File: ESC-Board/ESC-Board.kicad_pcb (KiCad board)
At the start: 2 copper layers, 17.1 x 32 mm, 26 parts, among them J1 Molex, J2 Molex, J3 XT_60, U1 ESC:Blue_ESC, U2 ESC:Blue_ESC, U3 ESC:Blue_ESC, U4 ESC:Blue_ESC

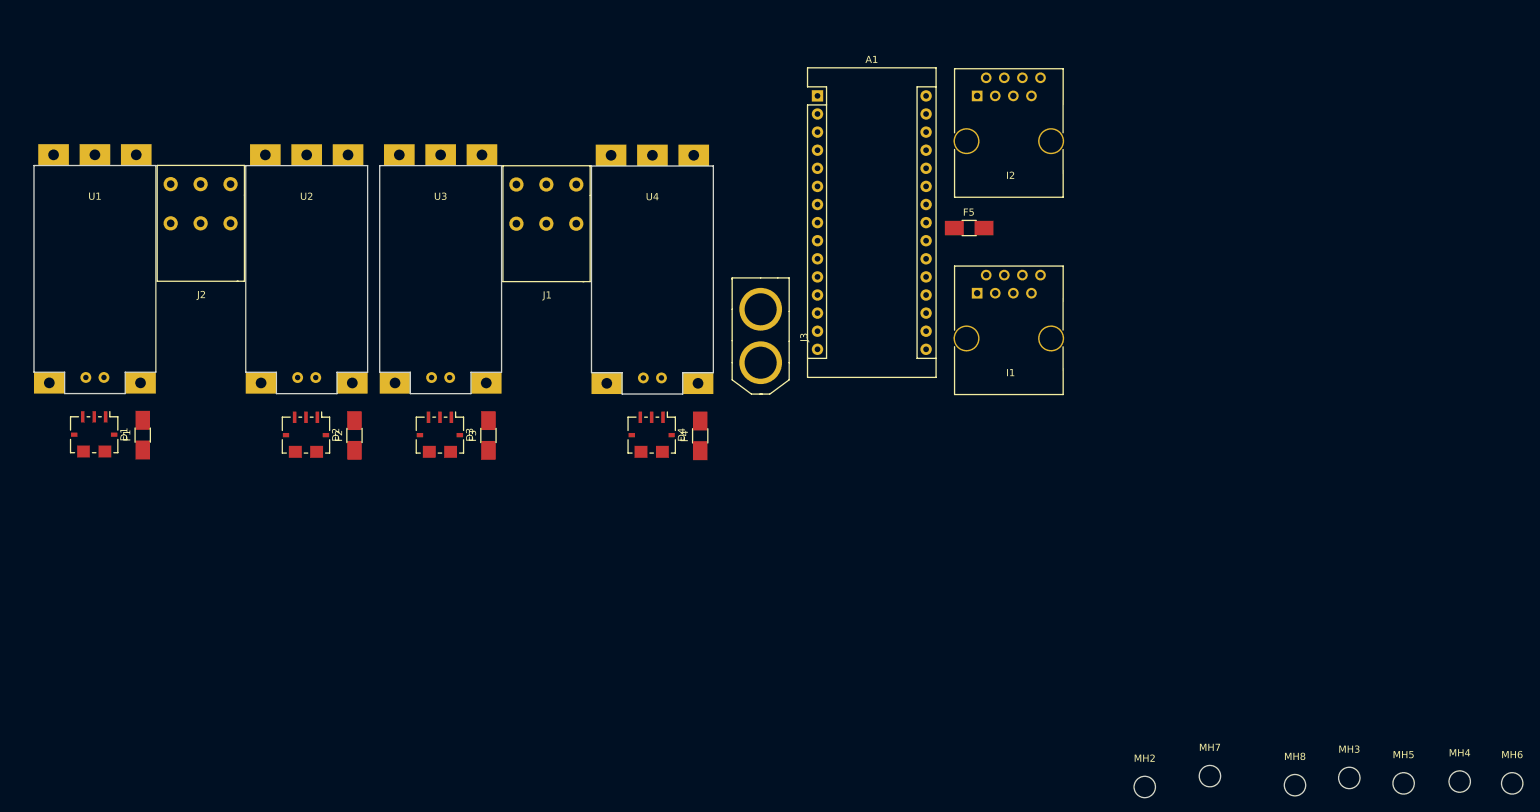
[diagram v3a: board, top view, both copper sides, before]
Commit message: I hate myself
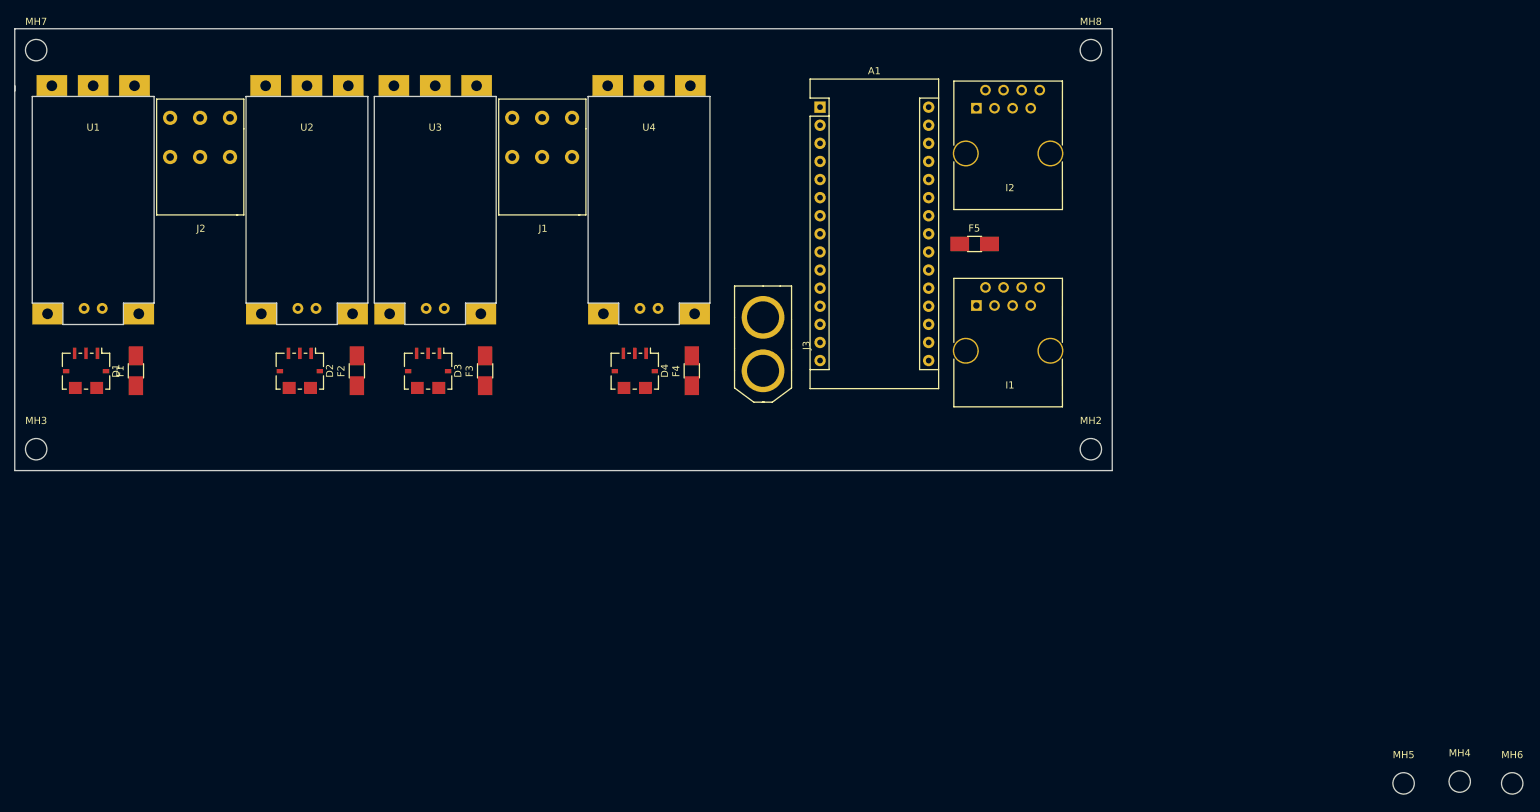
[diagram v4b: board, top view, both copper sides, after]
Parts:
- moved MH7 193.7 mm to (39.0, 49.0)
- moved MH3 190.0 mm to (39.0, 105.0)
- moved MH8 107.0 mm to (187.0, 49.0)
- moved MH2 48.0 mm to (187.0, 105.0)
- moved U4 9.77 mm to (125.0, 70.0)
- moved U3 9.73 mm to (95.0, 70.0)
- moved U2 9.71 mm to (77.0, 70.0)
- moved U1 9.70 mm to (47.0, 70.0)
- moved J1 9.37 mm to (110.0, 64.0)
- moved J2 9.30 mm to (62.0, 64.0)
- moved D4 9.28 mm to (123.0, 94.0)
- moved F4 9.20 mm to (131.0, 94.0)
- moved D3 9.12 mm to (94.0, 94.0)
- moved F3 9.09 mm to (102.0, 94.0)
- moved F2 9.08 mm to (84.0, 94.0)
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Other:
- board size 17.1 x 32 mm -> 154 x 62 mm
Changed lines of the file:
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@@
   (general
     (thickness 1.6)
-    (drawings 0)
+    (drawings 5)
     (tracks 0)
     (zones 0)
@@
     (add_net Power_ESC_4)
   )
+  (module Fuse_Holders_and_Fuses:Fuse_SMD1206_HandSoldering (layer F.Cu)
+    (at 84 94 90)
+    (descr "Fuse, Sicherung, SMD1206, Littlefuse-Wickmann 433 Series, Hand Soldering,")
+    (tags "Fuse Sicherung SMD1206 Littlefuse-Wickmann 433 Series Hand Soldering ")
+    (attr smd)
+    (fp_text reference F2 (at -0.05 -2.2 90) (layer F.SilkS)
+      (effects (font (size 1 1) (thickness 0.15)))
+    )
+    (fp_text value 10/15 (at -0.15 2.5 90) (layer F.Fab)
+      (effects (font (size 1 1) (thickness 0.15)))
+    )
+    (fp_line (start 3.35 1.58) (end -3.35 1.58) (layer F.CrtYd) (width 0.05))
+    (fp_line (start 3.35 1.58) (end 3.35 -1.58) (layer F.CrtYd) (width 0.05))
+    (fp_line (start -3.35 -1.58) (end -3.35 1.58) (layer F.CrtYd) (width 0.05))
+    (fp_line (start -3.35 -1.58) (end 3.35 -1.58) (layer F.CrtYd) (width 0.05))
+    (fp_line (start -1 -1.07) (end 1 -1.07) (layer F.SilkS) (width 0.12))
+    (fp_line (start 1 1.07) (end -1 1.07) (layer F.SilkS) (width 0.12))
+    (fp_line (start -1.6 -0.8) (end 1.6 -0.8) (layer F.Fab) (width 0.1))
+    (fp_line (start 1.6 -0.8) (end 1.6 0.8) (layer F.Fab) (width 0.1))
+    (fp_line (start 1.6 0.8) (end -1.6 0.8) (layer F.Fab) (width 0.1))
+    (fp_line (start -1.6 0.8) (end -1.6 -0.8) (layer F.Fab) (width 0.1))
+    (pad 2 smd rect (at 2.09 0 180) (size 2.03 2.65) (layers F.Cu F.Paste F.Mask)
+      (net 23 +12V))
+    (pad 1 smd rect (at -2.09 0 180) (size 2.03 2.65) (layers F.Cu F.Paste F.Mask)
+      (net 12 "Net-(D2-Pad6)"))
+  )
   (module Blue_ESC:Allegro_PSOF-7_4.8x6.4mm_Pitch1.60mm (layer F.Cu)
-    (at 47.1424 102.9208 270)
+    (at 46 94 270)
     (descr "Allegro Microsystems PSOF-7, 4.8x6.4mm Body, 1.60mm Pitch (http://www.allegromicro.com/~/media/Files/Datasheets/ACS780-Datasheet.ashx)")
     (tags "Allegro PSOF-7")
@@
   )
   (module Blue_ESC:Allegro_PSOF-7_4.8x6.4mm_Pitch1.60mm (layer F.Cu)
-    (at 76.8604 102.9716 270)
+    (at 76 94 270)
     (descr "Allegro Microsystems PSOF-7, 4.8x6.4mm Body, 1.60mm Pitch (http://www.allegromicro.com/~/media/Files/Datasheets/ACS780-Datasheet.ashx)")
     (tags "Allegro PSOF-7")
@@
   )
   (module Blue_ESC:Allegro_PSOF-7_4.8x6.4mm_Pitch1.60mm (layer F.Cu)
-    (at 95.6564 102.9716 270)
+    (at 94 94 270)
     (descr "Allegro Microsystems PSOF-7, 4.8x6.4mm Body, 1.60mm Pitch (http://www.allegromicro.com/~/media/Files/Datasheets/ACS780-Datasheet.ashx)")
     (tags "Allegro PSOF-7")
@@
   )
   (module Blue_ESC:Allegro_PSOF-7_4.8x6.4mm_Pitch1.60mm (layer F.Cu)
-    (at 125.3744 102.9716 270)
+    (at 123 94 270)
     (descr "Allegro Microsystems PSOF-7, 4.8x6.4mm Body, 1.60mm Pitch (http://www.allegromicro.com/~/media/Files/Datasheets/ACS780-Datasheet.ashx)")
     (tags "Allegro PSOF-7")
@@
   )
   (module Fuse_Holders_and_Fuses:Fuse_SMD1206_HandSoldering (layer F.Cu)
-    (at 53.9496 103.0224 90)
+    (at 53 94 90)
     (descr "Fuse, Sicherung, SMD1206, Littlefuse-Wickmann 433 Series, Hand Soldering,")
     (tags "Fuse Sicherung SMD1206 Littlefuse-Wickmann 433 Series Hand Soldering ")
@@
   )
   (module Fuse_Holders_and_Fuses:Fuse_SMD1206_HandSoldering (layer F.Cu)
-    (at 83.6676 103.0732 90)
-    (descr "Fuse, Sicherung, SMD1206, Littlefuse-Wickmann 433 Series, Hand Soldering,")
-    (tags "Fuse Sicherung SMD1206 Littlefuse-Wickmann 433 Series Hand Soldering ")
-    (attr smd)
-    (fp_text reference F2 (at -0.05 -2.2 90) (layer F.SilkS)
-      (effects (font (size 1 1) (thickness 0.15)))
-    )
-    (fp_text value 10/15 (at -0.15 2.5 90) (layer F.Fab)
-      (effects (font (size 1 1) (thickness 0.15)))
-    )
-    (fp_line (start 3.35 1.58) (end -3.35 1.58) (layer F.CrtYd) (width 0.05))
-    (fp_line (start 3.35 1.58) (end 3.35 -1.58) (layer F.CrtYd) (width 0.05))
-    (fp_line (start -3.35 -1.58) (end -3.35 1.58) (layer F.CrtYd) (width 0.05))
-    (fp_line (start -3.35 -1.58) (end 3.35 -1.58) (layer F.CrtYd) (width 0.05))
-    (fp_line (start -1 -1.07) (end 1 -1.07) (layer F.SilkS) (width 0.12))
-    (fp_line (start 1 1.07) (end -1 1.07) (layer F.SilkS) (width 0.12))
-    (fp_line (start -1.6 -0.8) (end 1.6 -0.8) (layer F.Fab) (width 0.1))
-    (fp_line (start 1.6 -0.8) (end 1.6 0.8) (layer F.Fab) (width 0.1))
-    (fp_line (start 1.6 0.8) (end -1.6 0.8) (layer F.Fab) (width 0.1))
-    (fp_line (start -1.6 0.8) (end -1.6 -0.8) (layer F.Fab) (width 0.1))
-    (pad 2 smd rect (at 2.09 0 180) (size 2.03 2.65) (layers F.Cu F.Paste F.Mask)
-      (net 23 +12V))
-    (pad 1 smd rect (at -2.09 0 180) (size 2.03 2.65) (layers F.Cu F.Paste F.Mask)
-      (net 12 "Net-(D2-Pad6)"))
-  )
-  (module Fuse_Holders_and_Fuses:Fuse_SMD1206_HandSoldering (layer F.Cu)
-    (at 102.4636 103.0732 90)
+    (at 102 94 90)
     (descr "Fuse, Sicherung, SMD1206, Littlefuse-Wickmann 433 Series, Hand Soldering,")
     (tags "Fuse Sicherung SMD1206 Littlefuse-Wickmann 433 Series Hand Soldering ")
@@
   )
   (module Fuse_Holders_and_Fuses:Fuse_SMD1206_HandSoldering (layer F.Cu)
-    (at 132.1816 103.124 90)
+    (at 131 94 90)
     (descr "Fuse, Sicherung, SMD1206, Littlefuse-Wickmann 433 Series, Hand Soldering,")
     (tags "Fuse Sicherung SMD1206 Littlefuse-Wickmann 433 Series Hand Soldering ")
@@
   )
   (module Fuse_Holders_and_Fuses:Fuse_SMD1206_HandSoldering (layer F.Cu)
-    (at 169.926 73.9648)
+    (at 170.688 76.2)
     (descr "Fuse, Sicherung, SMD1206, Littlefuse-Wickmann 433 Series, Hand Soldering,")
     (tags "Fuse Sicherung SMD1206 Littlefuse-Wickmann 433 Series Hand Soldering ")
@@
   )
   (module Connectors:RJ45_8 (layer F.Cu)
-    (at 171.0436 83.1088)
+    (at 170.942 84.836)
     (tags RJ45)
     (fp_text reference I1 (at 4.7 11.18) (layer F.SilkS)
@@
   )
   (module Connectors:RJ45_8 (layer F.Cu)
-    (at 171.0436 55.4228)
+    (at 170.942 57.15)
     (tags RJ45)
     (fp_text reference I2 (at 4.7 11.18) (layer F.SilkS)
@@
   )
   (module Blue_ESC:Molex_6pin (layer F.Cu)
-    (at 110.5916 73.3552)
+    (at 110 64)
     (fp_text reference J1 (at 0.127 10.033) (layer F.SilkS)
       (effects (font (size 1 1) (thickness 0.15)))
@@
   )
   (module Blue_ESC:Molex_6pin (layer F.Cu)
-    (at 62.0776 73.3044)
+    (at 62 64)
     (fp_text reference J2 (at 0.127 10.033) (layer F.SilkS)
       (effects (font (size 1 1) (thickness 0.15)))
@@
   )
   (module Blue_ESC:XT60 (layer F.Cu)
-    (at 140.6652 92.8624 90)
+    (at 141 94 90)
     (fp_text reference J3 (at 3.556 6.096 90) (layer F.SilkS)
       (effects (font (size 1 1) (thickness 0.15)))
@@
   )
   (module Mounting_Holes:MountingHole_3mm (layer F.Cu)
-    (at 194.564 152.4)
+    (at 187 105)
     (descr "Mounting Hole 3mm, no annular")
     (tags "mounting hole 3mm no annular")
@@
   )
   (module Mounting_Holes:MountingHole_3mm (layer F.Cu)
-    (at 223.266 151.13)
+    (at 39 105)
     (descr "Mounting Hole 3mm, no annular")
     (tags "mounting hole 3mm no annular")
@@
   )
   (module Mounting_Holes:MountingHole_3mm (layer F.Cu)
-    (at 203.708 150.876)
+    (at 39 49)
     (descr "Mounting Hole 3mm, no annular")
     (tags "mounting hole 3mm no annular")
@@
   )
   (module Mounting_Holes:MountingHole_3mm (layer F.Cu)
-    (at 215.646 152.146)
+    (at 187 49)
     (descr "Mounting Hole 3mm, no annular")
     (tags "mounting hole 3mm no annular")
@@
   )
   (module Blue_ESC:Blue_ESC (layer F.Cu)
-    (at 47.244 79.6925 180)
+    (at 47 70 180)
     (fp_text reference U1 (at 0 10.16 180) (layer F.SilkS)
       (effects (font (size 1 1) (thickness 0.15)))
@@
   )
   (module Blue_ESC:Blue_ESC (layer F.Cu)
-    (at 76.962 79.7052 180)
+    (at 77 70 180)
     (fp_text reference U2 (at 0 10.16 180) (layer F.SilkS)
       (effects (font (size 1 1) (thickness 0.15)))
@@
   )
   (module Blue_ESC:Blue_ESC (layer F.Cu)
-    (at 95.758 79.7052 180)
+    (at 95 70 180)
     (fp_text reference U3 (at 0 10.16 180) (layer F.SilkS)
       (effects (font (size 1 1) (thickness 0.15)))
@@
   )
   (module Blue_ESC:Blue_ESC (layer F.Cu)
-    (at 125.476 79.756 180)
+    (at 125 70 180)
     (fp_text reference U4 (at 0 10.16 180) (layer F.SilkS)
       (effects (font (size 1 1) (thickness 0.15)))
@@
   )
   (module Blue_ESC:Arduino_Nano (layer F.Cu)
-    (at 148.6408 55.4228)
+    (at 149 57)
     (descr "Arduino Nano, http://www.mouser.com/pdfdocs/Gravitech_Arduino_Nano3_0.pdf")
     (tags "Arduino Nano")
@@
     )
   )
+  (gr_line (start 36 46) (end 36 54.7376) (layer Edge.Cuts) (width 0.15))
+  (gr_line (start 36 108) (end 36 54) (layer Edge.Cuts) (width 0.15))
+  (gr_line (start 190 108) (end 36 108) (layer Edge.Cuts) (width 0.15))
+  (gr_line (start 189.992 46) (end 36 46) (layer Edge.Cuts) (width 0.15))
+  (gr_line (start 190 108) (end 190 46) (layer Edge.Cuts) (width 0.15))
 )

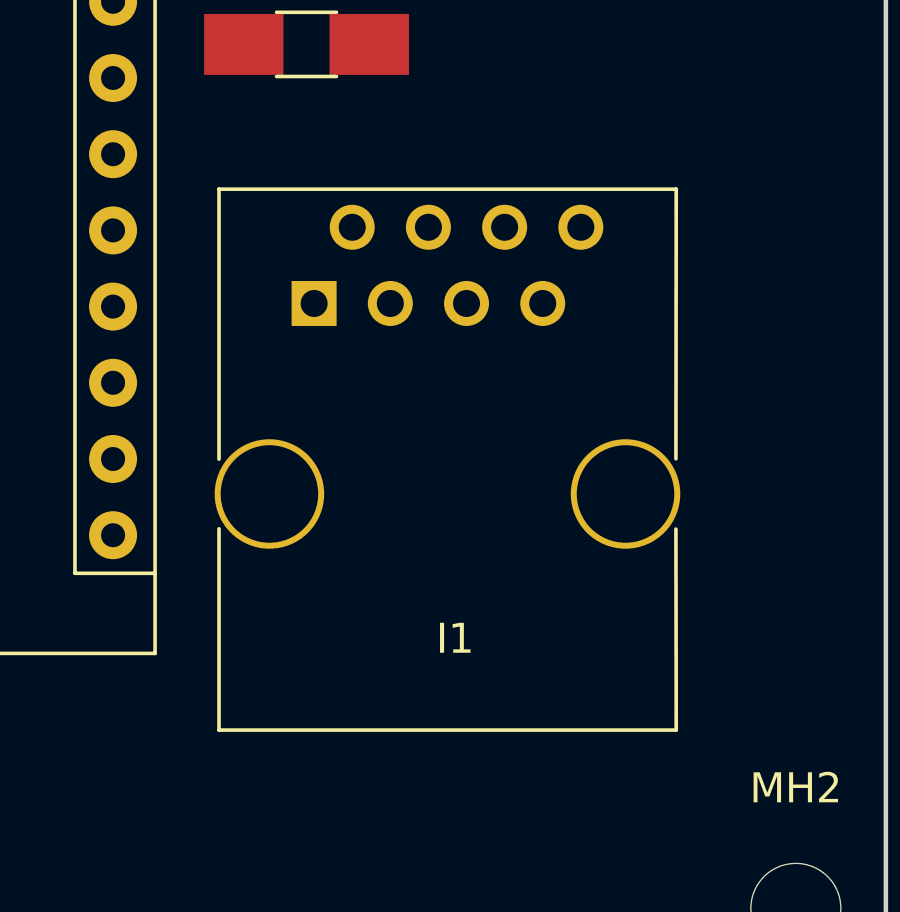
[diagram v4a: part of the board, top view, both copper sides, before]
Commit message: OOOF
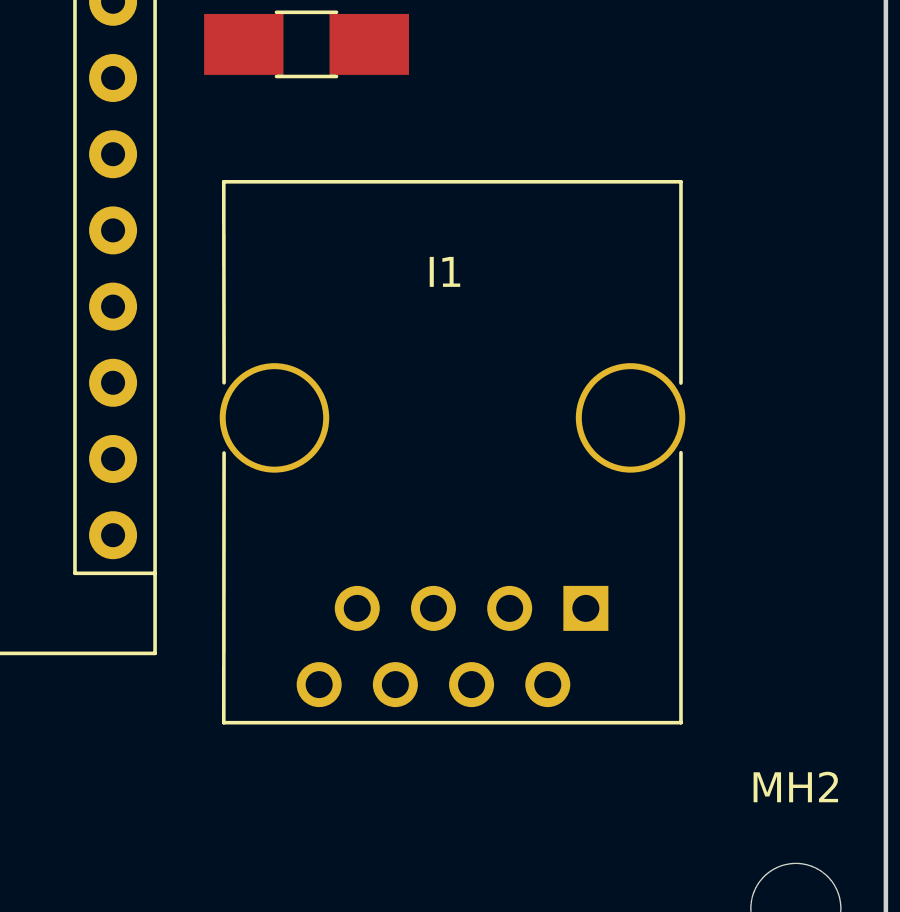
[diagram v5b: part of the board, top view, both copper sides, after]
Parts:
- moved I1 13.6 mm to (180.0, 95.0), turned to 180 degrees
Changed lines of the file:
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@@
   )
   (module Connectors:RJ45_8 (layer F.Cu)
-    (at 170.942 84.836)
+    (at 180 95 180)
     (tags RJ45)
-    (fp_text reference I1 (at 4.7 11.18) (layer F.SilkS)
+    (fp_text reference I1 (at 4.7 11.18 180) (layer F.SilkS)
       (effects (font (size 1 1) (thickness 0.15)))
     )
-    (fp_text value RJ45 (at 4.59 6.25) (layer F.Fab)
+    (fp_text value RJ45 (at 4.59 6.25 180) (layer F.Fab)
       (effects (font (size 1 1) (thickness 0.15)))
     )
@@
     (fp_line (start 12.07 -3.81) (end 12.06 5.18) (layer F.SilkS) (width 0.12))
     (fp_line (start -3.17 14.22) (end 12.07 14.22) (layer F.SilkS) (width 0.12))
-    (pad 8 thru_hole circle (at 8.89 -2.54) (size 1.5 1.5) (drill 0.9) (layers *.Cu *.Mask)
+    (pad 8 thru_hole circle (at 8.89 -2.54 180) (size 1.5 1.5) (drill 0.9) (layers *.Cu *.Mask)
       (net 25 "Net-(I1-Pad8)"))
-    (pad 7 thru_hole circle (at 7.62 0) (size 1.5 1.5) (drill 0.9) (layers *.Cu *.Mask)
+    (pad 7 thru_hole circle (at 7.62 0 180) (size 1.5 1.5) (drill 0.9) (layers *.Cu *.Mask)
       (net 26 "Net-(I1-Pad7)"))
-    (pad 6 thru_hole circle (at 6.35 -2.54) (size 1.5 1.5) (drill 0.9) (layers *.Cu *.Mask)
+    (pad 6 thru_hole circle (at 6.35 -2.54 180) (size 1.5 1.5) (drill 0.9) (layers *.Cu *.Mask)
       (net 27 "Net-(I1-Pad6)"))
-    (pad 5 thru_hole circle (at 5.08 0) (size 1.5 1.5) (drill 0.9) (layers *.Cu *.Mask)
+    (pad 5 thru_hole circle (at 5.08 0 180) (size 1.5 1.5) (drill 0.9) (layers *.Cu *.Mask)
       (net 28 "Net-(I1-Pad5)"))
-    (pad 4 thru_hole circle (at 3.81 -2.54) (size 1.5 1.5) (drill 0.9) (layers *.Cu *.Mask)
+    (pad 4 thru_hole circle (at 3.81 -2.54 180) (size 1.5 1.5) (drill 0.9) (layers *.Cu *.Mask)
       (net 29 "Net-(I1-Pad4)"))
-    (pad 3 thru_hole circle (at 2.54 0) (size 1.5 1.5) (drill 0.9) (layers *.Cu *.Mask)
+    (pad 3 thru_hole circle (at 2.54 0 180) (size 1.5 1.5) (drill 0.9) (layers *.Cu *.Mask)
       (net 6 GND))
-    (pad 2 thru_hole circle (at 1.27 -2.54) (size 1.5 1.5) (drill 0.9) (layers *.Cu *.Mask)
+    (pad 2 thru_hole circle (at 1.27 -2.54 180) (size 1.5 1.5) (drill 0.9) (layers *.Cu *.Mask)
       (net 30 I2C_SLC))
-    (pad 1 thru_hole rect (at 0 0) (size 1.5 1.5) (drill 0.9) (layers *.Cu *.Mask)
+    (pad 1 thru_hole rect (at 0 0 180) (size 1.5 1.5) (drill 0.9) (layers *.Cu *.Mask)
       (net 31 I2C_SDA))
-    (pad Hole np_thru_hole circle (at -1.49 6.35) (size 3.65 3.65) (drill 3.25) (layers *.Cu *.SilkS *.Mask))
-    (pad Hole np_thru_hole circle (at 10.38 6.35) (size 3.65 3.65) (drill 3.25) (layers *.Cu *.SilkS *.Mask))
+    (pad Hole np_thru_hole circle (at -1.49 6.35 180) (size 3.65 3.65) (drill 3.25) (layers *.Cu *.SilkS *.Mask))
+    (pad Hole np_thru_hole circle (at 10.38 6.35 180) (size 3.65 3.65) (drill 3.25) (layers *.Cu *.SilkS *.Mask))
     (model ${KISYS3DMOD}/Connectors.3dshapes/RJ45_8.wrl
       (offset (xyz 4.571999931335449 -6.349999904632568 0))
